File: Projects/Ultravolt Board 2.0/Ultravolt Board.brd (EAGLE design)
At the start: 65.4 x 30.5 mm, 8 parts

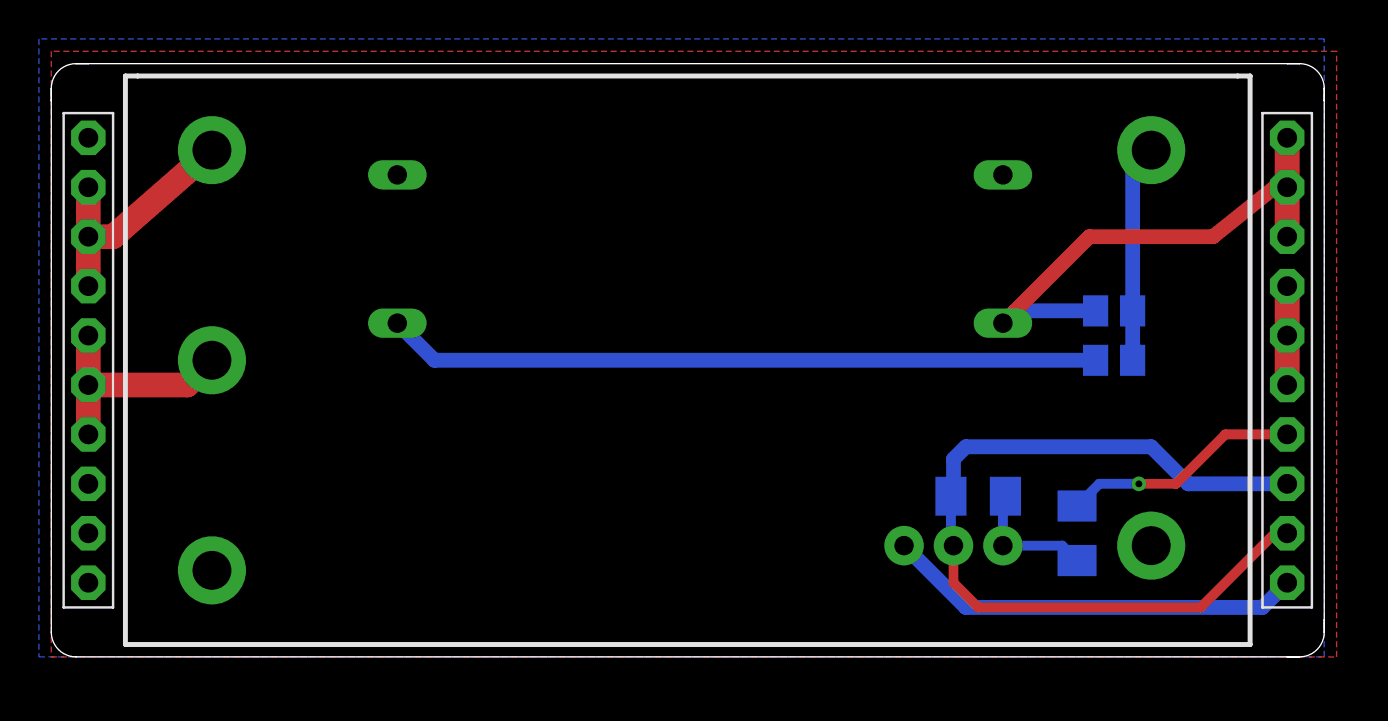
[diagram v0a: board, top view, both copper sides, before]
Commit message: Update with Microphones
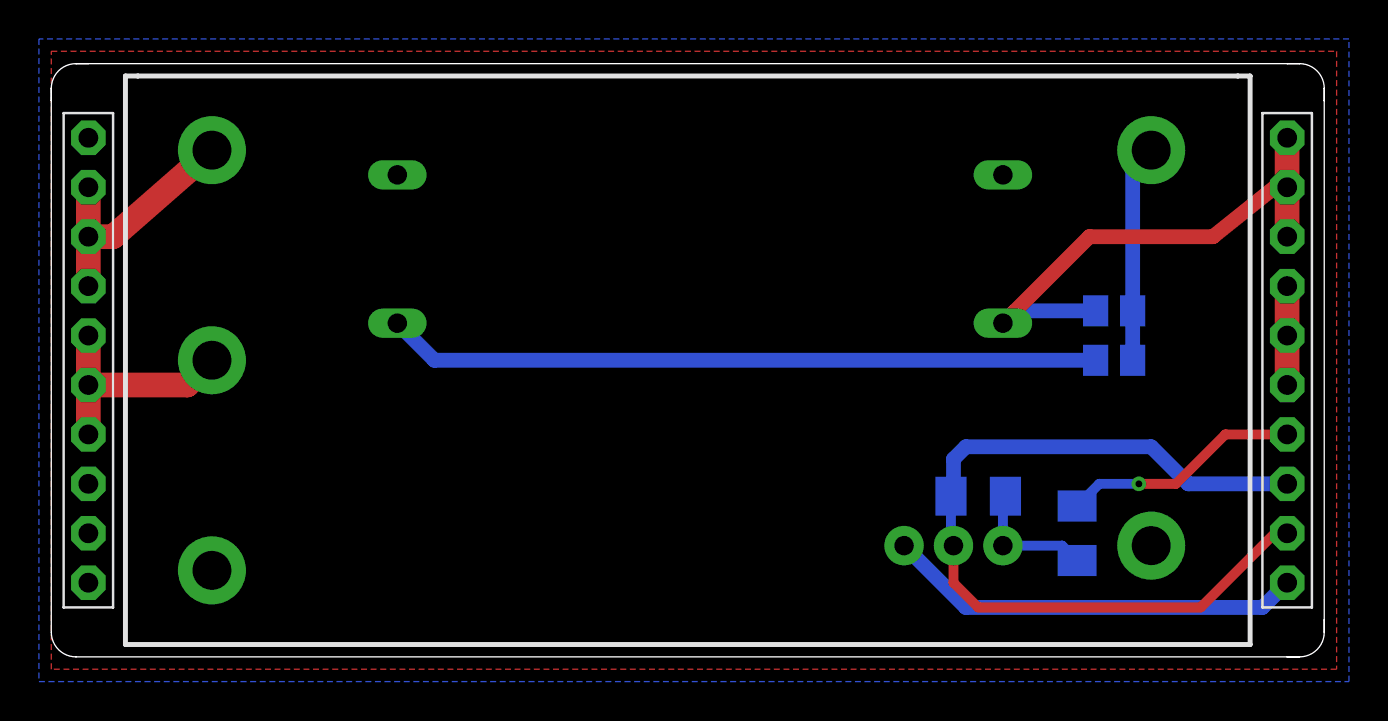
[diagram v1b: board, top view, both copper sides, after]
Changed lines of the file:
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@@
 <?xml version="1.0" encoding="utf-8"?>
 <!DOCTYPE eagle SYSTEM "eagle.dtd">
-<eagle version="9.0.1">
+<eagle version="9.1.1">
 <drawing>
 <settings>
-<setting alwaysvectorfont="no"/>
+<setting alwaysvectorfont="yes"/>
 <setting verticaltext="up"/>
 </settings>
@@
 <wire x1="52.07" y1="29.845" x2="14.605" y2="29.845" width="0.254" layer="22"/>
 <text x="26.035" y="27.94" size="0.254" layer="22" rot="MR0">[Potentiometer]</text>
-<text x="33.02" y="9.525" size="0.254" layer="22" rot="MR0">Lucas Mun 2018</text>
-<text x="34.925" y="8.255" size="0.254" layer="22" rot="MR0">HV-DC Converter Board - Ultravolt RS series</text>
+<text x="33.02" y="9.525" size="1.016" layer="22" rot="MR0">Lucas Mun 2018</text>
+<text x="34.925" y="8.255" size="1.016" layer="22" rot="MR0">HV-DC Converter Board - Ultravolt RS series</text>
+<dimension x1="0" y1="-0.635" x2="65.405" y2="-0.635" x3="32.7025" y3="-6.35" textsize="1.778" layer="1"/>
+<dimension x1="66.04" y1="-0.635" x2="66.04" y2="30.48" x3="71.12" y3="14.9225" textsize="1.778" layer="1"/>
 </plain>
 <attributes>
@@
 <param name="checkStop" value="0"/>
 <param name="checkValues" value="0"/>
+<param name="checkNames" value="1"/>
+<param name="checkWireStubs" value="1"/>
+<param name="checkPolygonWidth" value="0"/>
 <param name="useDiameter" value="13"/>
 <param name="maxErrors" value="50"/>
@@
 <wire x1="63.5" y1="19.05" x2="63.5" y2="16.51" width="1.27" layer="1"/>
 <wire x1="63.5" y1="16.51" x2="63.5" y2="13.97" width="1.27" layer="1"/>
-<polygon width="0.0254" layer="16">
+<polygon width="0.1524" layer="16">
+<vertex x="-0.635" y="-1.27"/>
+<vertex x="66.675" y="-1.27"/>
+<vertex x="66.675" y="31.75"/>
 <vertex x="-0.635" y="31.75"/>
-<vertex x="-0.635" y="0"/>
-<vertex x="65.405" y="0"/>
-<vertex x="65.405" y="31.75"/>
 </polygon>
-<polygon width="0.0254" layer="1">
-<vertex x="0" y="0"/>
-<vertex x="66.04" y="0"/>
+<polygon width="0.1524" layer="1">
 <vertex x="66.04" y="31.115"/>
+<vertex x="66.04" y="-0.635"/>
+<vertex x="0" y="-0.635"/>
 <vertex x="0" y="31.115"/>
 </polygon>
@@
 </signal>
 </signals>
+<mfgpreviewcolors>
+<mfgpreviewcolor name="soldermaskcolor" color="0xC8008000"/>
+<mfgpreviewcolor name="silkscreencolor" color="0xFFFEFEFE"/>
+<mfgpreviewcolor name="backgroundcolor" color="0xFF282828"/>
+<mfgpreviewcolor name="coppercolor" color="0xFFFFBF00"/>
+<mfgpreviewcolor name="substratecolor" color="0xFF786E46"/>
+</mfgpreviewcolors>
 </board>
 </drawing>
